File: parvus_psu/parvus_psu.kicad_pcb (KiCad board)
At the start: 2 copper layers, 100 x 100 mm, 67 parts, among them J1 tr_sec, J2 switch, J3 ac_input, J4 tr_pri, J5 power_1, J6 power_2, J7 signal, J8 ctrl_1, J9 ctrl_2, Q1 BC546B, Q2 BC546B, Q3 BC546B, Q4 BC546B, Q5 BC546B, Q6 BC556B, Q7 BC556B, Q8 BC556B

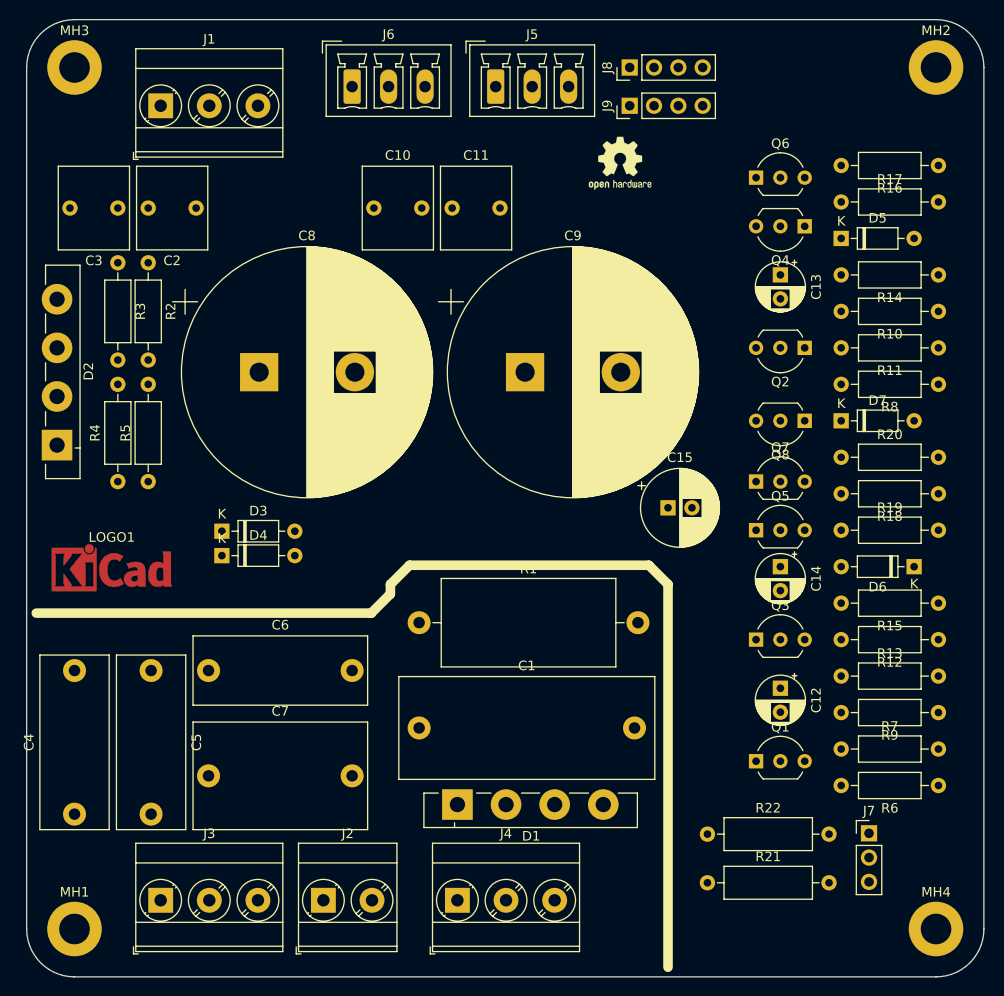
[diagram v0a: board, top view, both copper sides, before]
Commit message: Updated to new version v1.02.
Signed-off-by: Nenad Radulovic <nenad.b.radulovic@gmail.com>
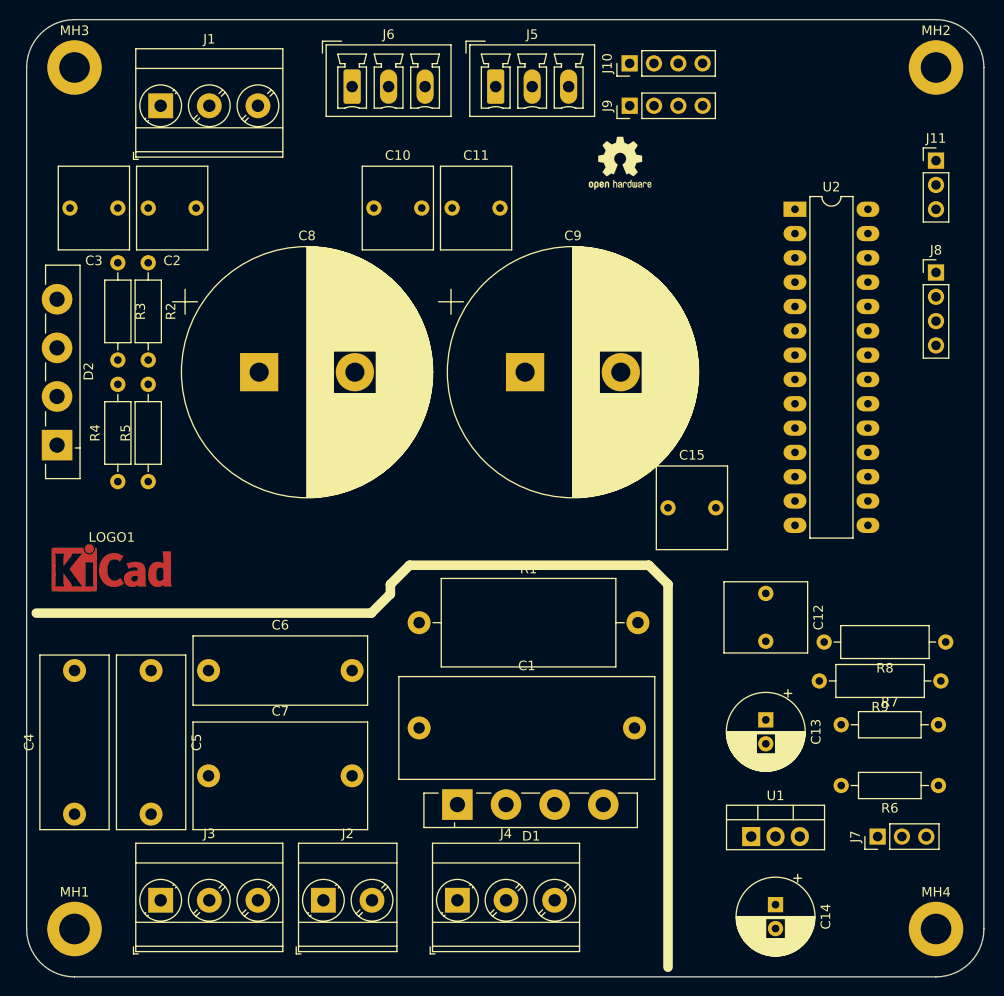
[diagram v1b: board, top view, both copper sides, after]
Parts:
- removed D3, D4, D5, D6, D7: 1N4148, Diode_THT:D_DO-35_SOD27_P7.62mm_Horizontal
- removed Q1, Q2, Q3, Q4, Q5: BC546B, Package_TO_SOT_THT:TO-92_Inline_Wide
- removed Q6, Q7, Q8: BC556B, Package_TO_SOT_THT:TO-92_Inline_Wide
- removed R10, R12, R14, R15: 100k, Resistor_THT:R_Axial_DIN0207_L6.3mm_D2.5mm_P10.16mm_Horizontal
- removed R11, R13: 100, Resistor_THT:R_Axial_DIN0207_L6.3mm_D2.5mm_P10.16mm_Horizontal
- removed R16, R17, R18, R19, R20: 22k, Resistor_THT:R_Axial_DIN0207_L6.3mm_D2.5mm_P10.16mm_Horizontal
- removed R21, R22: 4k7, Resistor_THT:R_Axial_DIN0309_L9.0mm_D3.2mm_P12.70mm_Horizontal
- added J10: ctrl_2, Connector_PinHeader_2.54mm:PinHeader_1x04_P2.54mm_Vertical, F.Cu at (123.0, 44.6)
- added J11: signal, Connector_PinHeader_2.54mm:PinHeader_1x03_P2.54mm_Vertical, F.Cu at (155.0, 54.7)
- added U1: L7805, Package_TO_SOT_THT:TO-220-3_Vertical, F.Cu at (135.7, 125.3)
- added U2: PIC18F26K20_ISS, Package_DIP:DIP-28_W7.62mm_LongPads, F.Cu at (140.3, 59.8)
- C12: value 2u2 -> 470n; footprint Capacitor_THT:CP_Radial_D5.0mm_P2.50mm -> Capacitor_THT:C_Rect_L7.2mm_W8.5mm_P5.00mm_FKP2_FKP2_MKS2_MKP2
- C13: value 4u7 -> 10u; footprint Capacitor_THT:CP_Radial_D5.0mm_P2.50mm -> Capacitor_THT:CP_Radial_D8.0mm_P2.50mm
- C14: value 2u2 -> 10u; footprint Capacitor_THT:CP_Radial_D5.0mm_P2.50mm -> Capacitor_THT:CP_Radial_D8.0mm_P2.50mm
- C15: value 10u -> 470n; footprint Capacitor_THT:CP_Radial_D8.0mm_P2.50mm -> Capacitor_THT:C_Rect_L7.2mm_W8.5mm_P5.00mm_FKP2_FKP2_MKS2_MKP2
- J8: value ctrl_1 -> prog
- J9: value ctrl_2 -> ctrl_1
- R7: value 10k -> 100k
- R8: value 47k -> 1k; footprint Resistor_THT:R_Axial_DIN0207_L6.3mm_D2.5mm_P10.16mm_Horizontal -> Resistor_THT:R_Axial_DIN0309_L9.0mm_D3.2mm_P12.70mm_Horizontal
- R9: value 100k -> 1k; footprint Resistor_THT:R_Axial_DIN0207_L6.3mm_D2.5mm_P10.16mm_Horizontal -> Resistor_THT:R_Axial_DIN0309_L9.0mm_D3.2mm_P12.70mm_Horizontal
- moved C13 46.5 mm to (137.2, 113.2)
- moved J8 38.5 mm to (155.0, 66.4), turned to 0 degrees
- moved C14 35.3 mm to (138.2, 132.5)
- moved R8 26.9 mm to (156.0, 105.0)
- moved C12 10.0 mm to (137.2, 99.9)
- moved R9 3.31 mm to (155.5, 109.1)
- moved R7 2.54 mm to (145.1, 113.7)
- moved J7 0.96 mm to (148.9, 125.3), turned to 90 degrees
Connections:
- C13 pad 1: Net-(C13-Pad1) -> /vcc
- C14 pad 1: Net-(C14-Pad1) -> vdd
- C15 pad 1: /vcc -> vdd
- J8 pad 1: (no net) -> vdd
- J8 pad 2: /mute_control -> Net-(J8-Pad2)
- J8 pad 4: /clipping -> Net-(J8-Pad4)
- R6 pad 1: Net-(D3-Pad1) -> acs_p
- R6 pad 2: Net-(Q1-Pad2) -> /ac_detect
- R7 pad 1: Net-(Q1-Pad2) -> vdd
- R7 pad 2: GNDPWR -> Net-(J8-Pad2)
- R8 pad 1: /vcc -> Net-(J7-Pad3)
- R8 pad 2: /clipping -> Net-(R8-Pad2)
- R9 pad 1: /vcc -> Net-(J7-Pad1)
- R9 pad 2: /ac_detect -> Net-(R9-Pad2)

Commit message: Project update
Signed-off-by: Nenad Radulovic <nenad.b.radulovic@gmail.com>
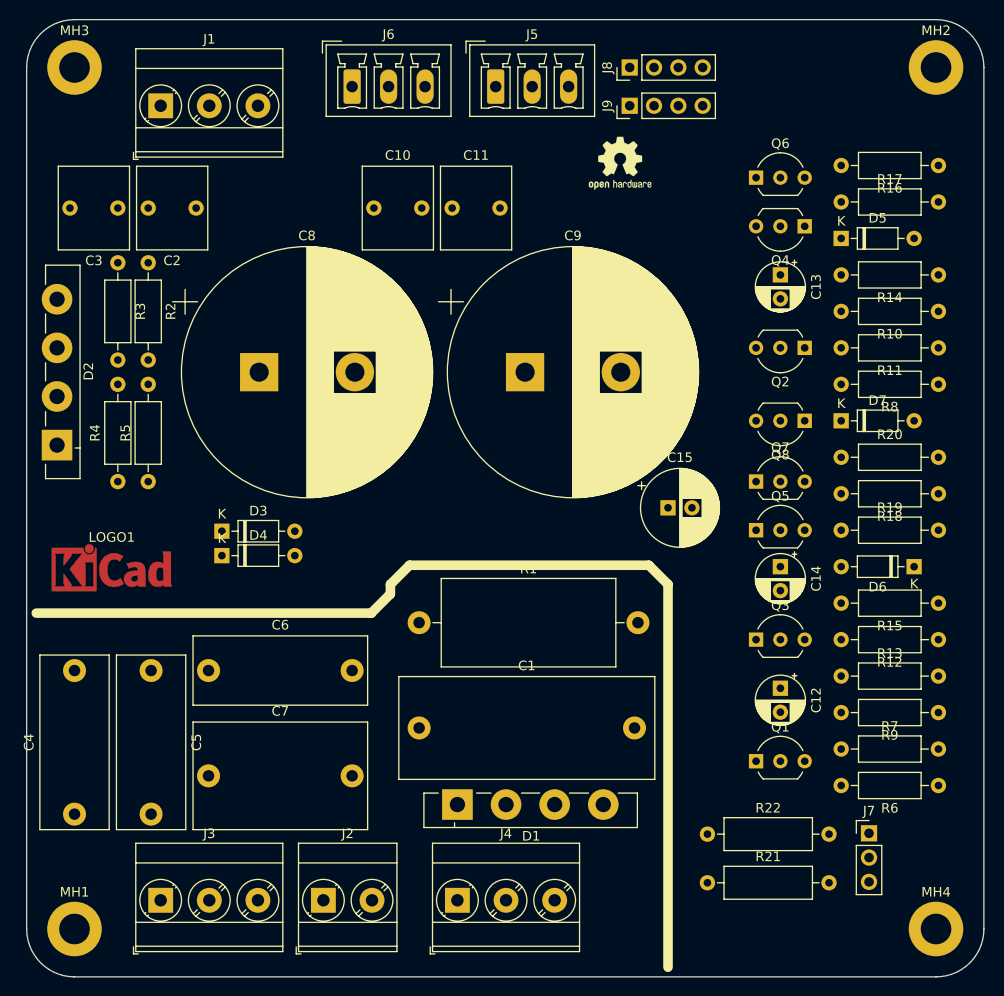
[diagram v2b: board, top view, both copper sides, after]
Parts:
- removed J10: ctrl_2, Connector_PinHeader_2.54mm:PinHeader_1x04_P2.54mm_Vertical
- removed J11: signal, Connector_PinHeader_2.54mm:PinHeader_1x03_P2.54mm_Vertical
- removed U1: L7805, Package_TO_SOT_THT:TO-220-3_Vertical
- removed U2: PIC18F26K20_ISS, Package_DIP:DIP-28_W7.62mm_LongPads
- added D3: 1N4148, Diode_THT:D_DO-35_SOD27_P7.62mm_Horizontal, F.Cu at (80.4, 93.4)
- added D4: 1N4148, Diode_THT:D_DO-35_SOD27_P7.62mm_Horizontal, F.Cu at (80.4, 96.0)
- added D5: 1N4148, Diode_THT:D_DO-35_SOD27_P7.62mm_Horizontal, F.Cu at (145.1, 62.9)
- added D6: 1N4148, Diode_THT:D_DO-35_SOD27_P7.62mm_Horizontal, F.Cu at (152.7, 97.2)
- added D7: 1N4148, Diode_THT:D_DO-35_SOD27_P7.62mm_Horizontal, F.Cu at (145.1, 81.9)
- added Q1: BC546B, Package_TO_SOT_THT:TO-92_Inline_Wide, F.Cu at (136.2, 117.5)
- added Q2: BC546B, Package_TO_SOT_THT:TO-92_Inline_Wide, F.Cu at (141.3, 74.3)
- added Q3: BC546B, Package_TO_SOT_THT:TO-92_Inline_Wide, F.Cu at (136.2, 104.8)
- added Q4: BC546B, Package_TO_SOT_THT:TO-92_Inline_Wide, F.Cu at (141.3, 61.6)
- added Q5: BC546B, Package_TO_SOT_THT:TO-92_Inline_Wide, F.Cu at (136.2, 93.3)
- added Q6: BC556B, Package_TO_SOT_THT:TO-92_Inline_Wide, F.Cu at (136.2, 56.5)
- added Q7: BC556B, Package_TO_SOT_THT:TO-92_Inline_Wide, F.Cu at (136.2, 88.3)
- added Q8: BC556B, Package_TO_SOT_THT:TO-92_Inline_Wide, F.Cu at (141.3, 81.9)
- added R10: 100k, Resistor_THT:R_Axial_DIN0207_L6.3mm_D2.5mm_P10.16mm_Horizontal, F.Cu at (155.2, 70.5)
- added R11: 100, Resistor_THT:R_Axial_DIN0207_L6.3mm_D2.5mm_P10.16mm_Horizontal, F.Cu at (155.2, 74.3)
- added R12: 100k, Resistor_THT:R_Axial_DIN0207_L6.3mm_D2.5mm_P10.16mm_Horizontal, F.Cu at (155.2, 104.8)
- added R13: 100, Resistor_THT:R_Axial_DIN0207_L6.3mm_D2.5mm_P10.16mm_Horizontal, F.Cu at (145.1, 108.6)
- added R14: 100k, Resistor_THT:R_Axial_DIN0207_L6.3mm_D2.5mm_P10.16mm_Horizontal, F.Cu at (155.2, 66.7)
- added R15: 100k, Resistor_THT:R_Axial_DIN0207_L6.3mm_D2.5mm_P10.16mm_Horizontal, F.Cu at (155.2, 101.0)
- added R16: 22k, Resistor_THT:R_Axial_DIN0207_L6.3mm_D2.5mm_P10.16mm_Horizontal, F.Cu at (155.2, 55.2)
- added R17: 22k, Resistor_THT:R_Axial_DIN0207_L6.3mm_D2.5mm_P10.16mm_Horizontal, F.Cu at (145.1, 59.0)
- added R18: 22k, Resistor_THT:R_Axial_DIN0207_L6.3mm_D2.5mm_P10.16mm_Horizontal, F.Cu at (155.2, 89.5)
- added R19: 22k, Resistor_THT:R_Axial_DIN0207_L6.3mm_D2.5mm_P10.16mm_Horizontal, F.Cu at (145.1, 93.3)
- added R20: 22k, Resistor_THT:R_Axial_DIN0207_L6.3mm_D2.5mm_P10.16mm_Horizontal, F.Cu at (145.1, 85.7)
- added R21: 4k7, Resistor_THT:R_Axial_DIN0309_L9.0mm_D3.2mm_P12.70mm_Horizontal, F.Cu at (131.1, 130.2)
- added R22: 4k7, Resistor_THT:R_Axial_DIN0309_L9.0mm_D3.2mm_P12.70mm_Horizontal, F.Cu at (131.1, 125.1)
- C12: value 470n -> 2u2; footprint Capacitor_THT:C_Rect_L7.2mm_W8.5mm_P5.00mm_FKP2_FKP2_MKS2_MKP2 -> Capacitor_THT:CP_Radial_D5.0mm_P2.50mm
- C13: value 10u -> 4u7; footprint Capacitor_THT:CP_Radial_D8.0mm_P2.50mm -> Capacitor_THT:CP_Radial_D5.0mm_P2.50mm
- C14: value 10u -> 2u2; footprint Capacitor_THT:CP_Radial_D8.0mm_P2.50mm -> Capacitor_THT:CP_Radial_D5.0mm_P2.50mm
- C15: value 470n -> 10u; footprint Capacitor_THT:C_Rect_L7.2mm_W8.5mm_P5.00mm_FKP2_FKP2_MKS2_MKP2 -> Capacitor_THT:CP_Radial_D8.0mm_P2.50mm
- J8: value prog -> ctrl_1
- J9: value ctrl_1 -> ctrl_2
- R7: value 100k -> 10k
- R8: value 1k -> 47k; footprint Resistor_THT:R_Axial_DIN0309_L9.0mm_D3.2mm_P12.70mm_Horizontal -> Resistor_THT:R_Axial_DIN0207_L6.3mm_D2.5mm_P10.16mm_Horizontal
- R9: value 1k -> 100k; footprint Resistor_THT:R_Axial_DIN0309_L9.0mm_D3.2mm_P12.70mm_Horizontal -> Resistor_THT:R_Axial_DIN0207_L6.3mm_D2.5mm_P10.16mm_Horizontal
- moved C13 46.5 mm to (138.7, 66.7)
- moved J8 38.5 mm to (123.0, 45.0), turned to 90 degrees
- moved C14 35.3 mm to (138.7, 97.2)
- moved R8 26.9 mm to (155.2, 78.1)
- moved C12 10.0 mm to (138.7, 109.8)
- moved R9 3.31 mm to (155.2, 112.4)
- moved R7 2.54 mm to (145.1, 116.2)
- moved J7 0.96 mm to (148.0, 125.0), turned to 0 degrees
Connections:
- C13 pad 1: /vcc -> Net-(C13-Pad1)
- C14 pad 1: vdd -> Net-(C14-Pad1)
- C15 pad 1: vdd -> /vcc
- J8 pad 1: vdd -> (no net)
- J8 pad 2: Net-(J8-Pad2) -> /mute_control
- J8 pad 4: Net-(J8-Pad4) -> /clipping
- R6 pad 1: acs_p -> Net-(D3-Pad1)
- R6 pad 2: /ac_detect -> Net-(Q1-Pad2)
- R7 pad 1: vdd -> Net-(Q1-Pad2)
- R7 pad 2: Net-(J8-Pad2) -> GNDPWR
- R8 pad 1: Net-(J7-Pad3) -> /vcc
- R8 pad 2: Net-(R8-Pad2) -> /clipping
- R9 pad 1: Net-(J7-Pad1) -> /vcc
- R9 pad 2: Net-(R9-Pad2) -> /ac_detect
